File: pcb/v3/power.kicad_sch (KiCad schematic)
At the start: 51 parts, among them J6 Conn_01x02, J7 Conn_01x02, J8 Conn_01x03, J9 Conn_01x02, Q1 NPN, Q2 NPN, Q3 PMOS, U2 LM27762, U3 SY6918QDC, U5 LP5912-3.3DRV

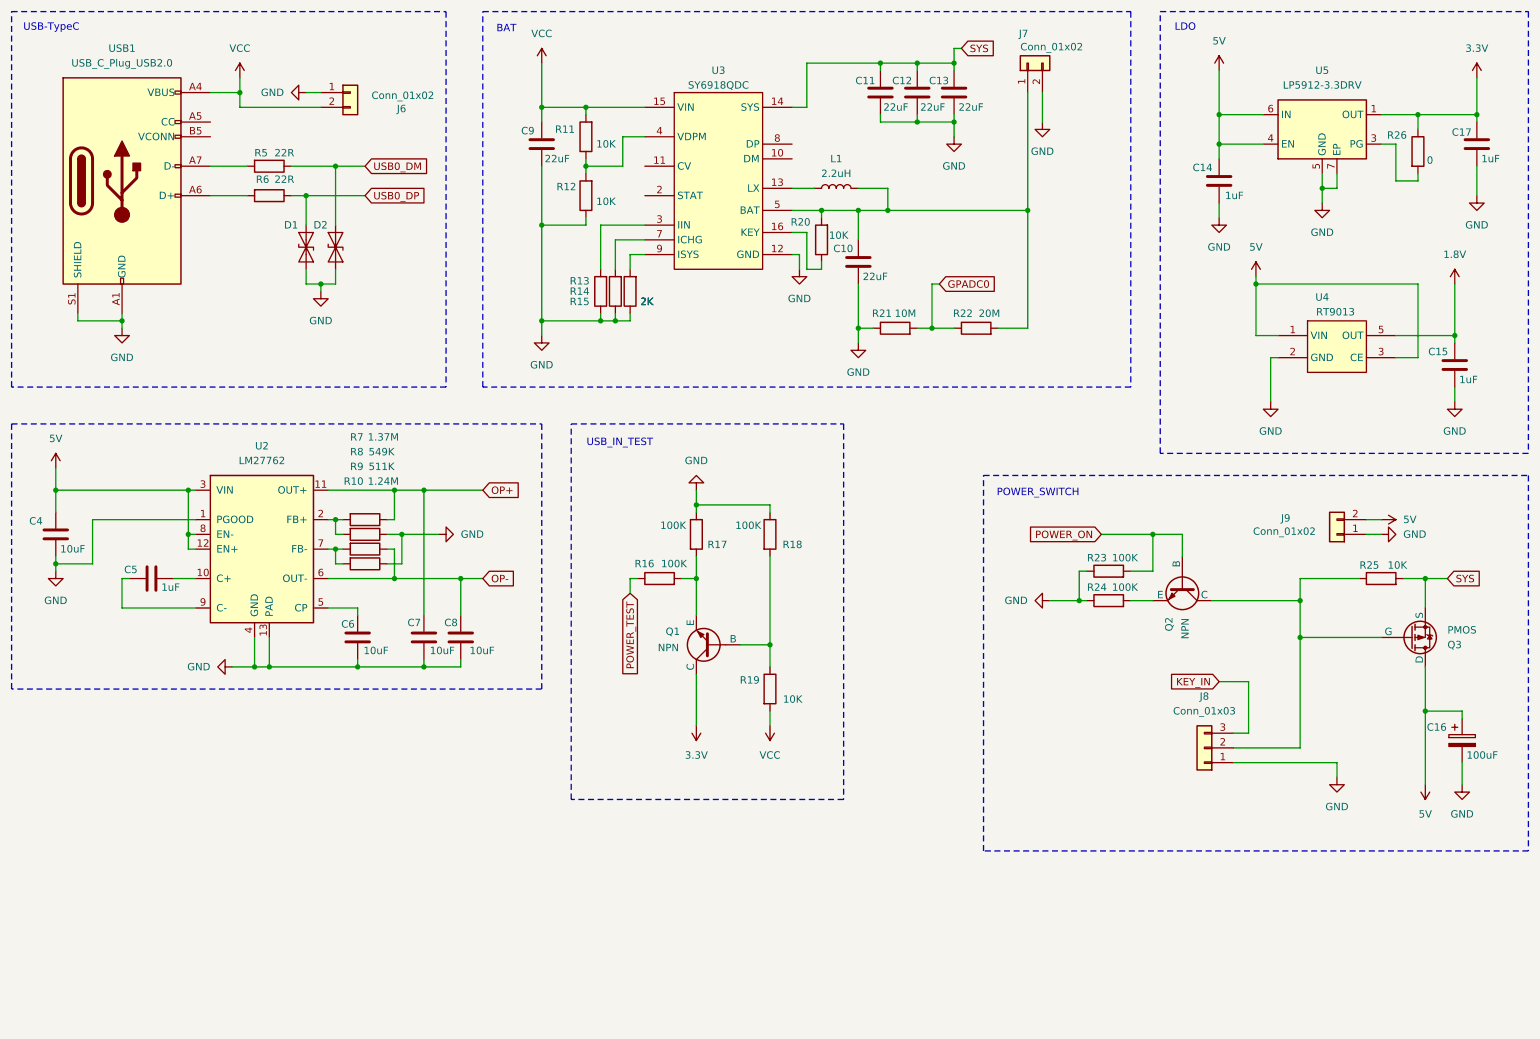
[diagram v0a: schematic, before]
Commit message: up
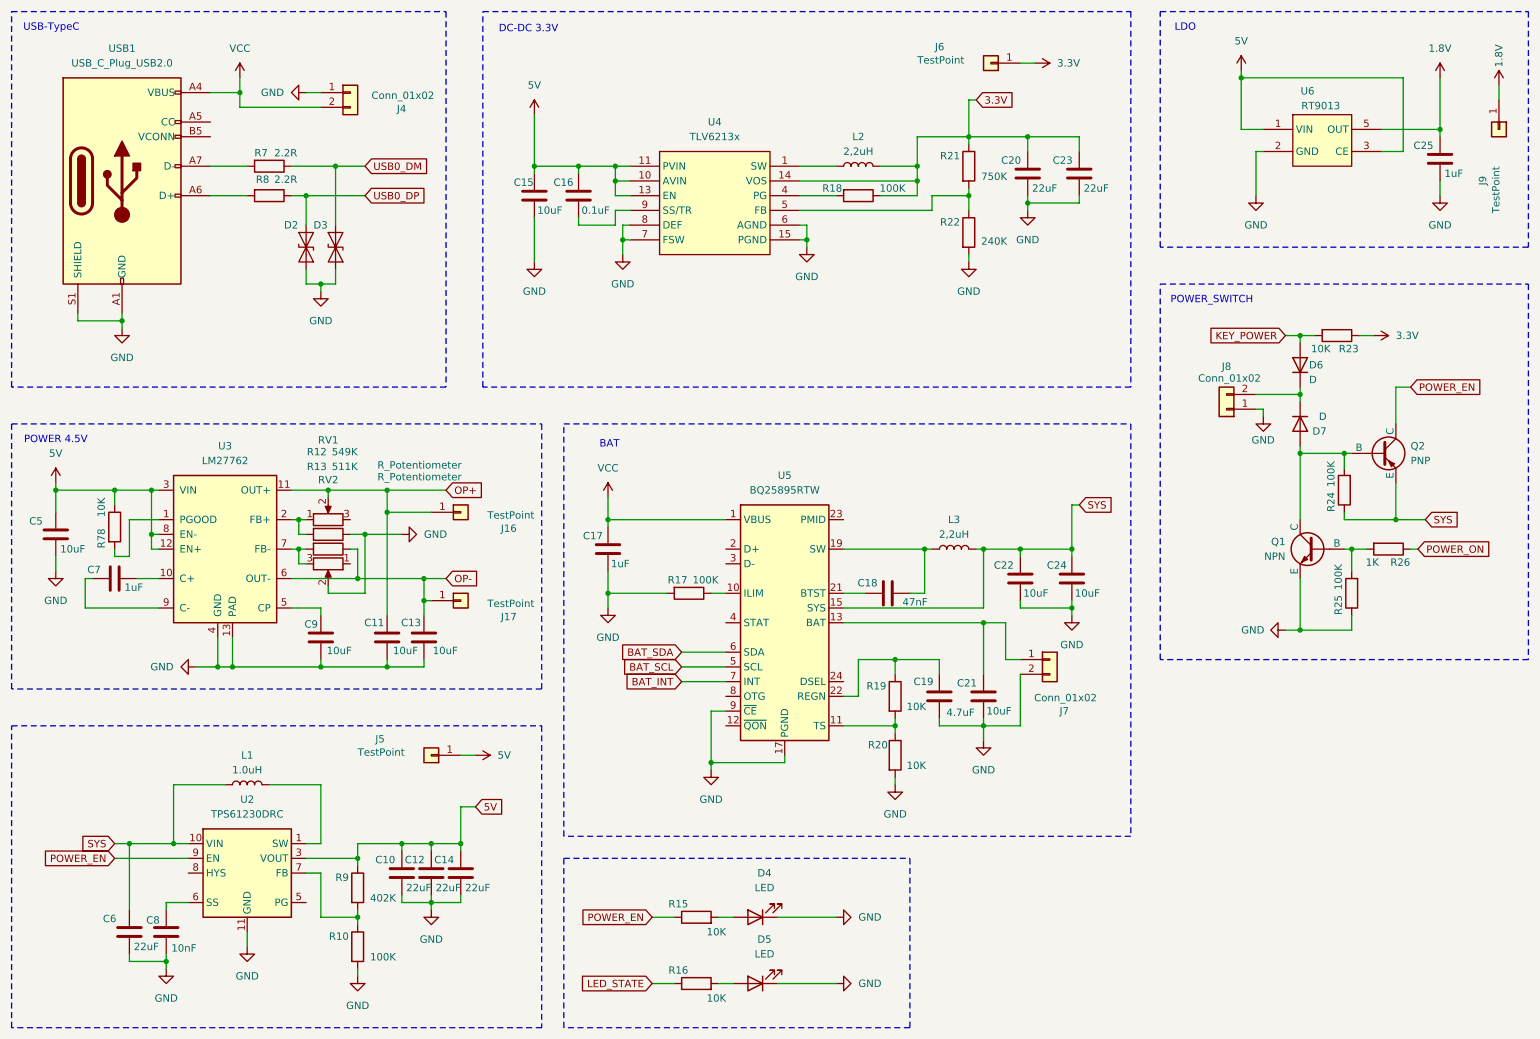
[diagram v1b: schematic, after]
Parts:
- removed C11, C13: 22uF, Capacitor_SMD:C_0603_1608Metric_Pad1.08x0.95mm_HandSolder, symbol Device:C
- removed C16: 100uF, Capacitor_Tantalum_SMD:CP_EIA-3528-21_Kemet-B_Pad1.50x2.35mm_HandSolder, symbol Device:C_Polarized
- removed Q2: NPN, Package_TO_SOT_SMD:SOT-23, symbol Simulation_SPICE:NPN
- removed Q3: PMOS, Package_TO_SOT_SMD:SOT-23_Handsoldering, symbol Simulation_SPICE:PMOS
- removed R11, R12: 10K, Capacitor_SMD:C_0402_1005Metric_Pad0.74x0.62mm_HandSolder, symbol Device:R
- removed R13, R14: 2K, Capacitor_SMD:C_0402_1005Metric_Pad0.74x0.62mm_HandSolder, symbol Device:R
- removed R7: 1.37M, Capacitor_SMD:C_0402_1005Metric_Pad0.74x0.62mm_HandSolder, symbol Device:R
- removed U3: SY6918QDC, coloryr:SY6918, symbol coloryr:SY6918
- removed U5: LP5912-3.3DRV, Package_SON:WSON-6-1EP_2x2mm_P0.65mm_EP1x1.6mm_ThermalVias, symbol Regulator_Linear:LP5912-3.3DRV
- added C16: 0.1uF, Capacitor_SMD:C_0402_1005Metric_Pad0.74x0.62mm_HandSolder, symbol Device:C
- added C18: 47nF, Capacitor_SMD:C_0402_1005Metric_Pad0.74x0.62mm_HandSolder, symbol Device:C
- added C19: 4.7uF, Capacitor_SMD:C_0402_1005Metric_Pad0.74x0.62mm_HandSolder, symbol Device:C
- added C20, C23: 22uF, Capacitor_SMD:C_0603_1608Metric_Pad1.08x0.95mm_HandSolder, symbol Device:C
- added C21, C22, C24: 10uF, Capacitor_SMD:C_0402_1005Metric_Pad0.74x0.62mm_HandSolder, symbol Device:C
- added C6: 22uF, Capacitor_SMD:C_0402_1005Metric_Pad0.74x0.62mm_HandSolder, symbol Device:C
- added C8: 10nF, Capacitor_SMD:C_0402_1005Metric_Pad0.74x0.62mm_HandSolder, symbol Device:C
- added D4, D5: LED, Diode_SMD:D_0402_1005Metric_Pad0.77x0.64mm_HandSolder, symbol Device:LED
- added D6, D7: D, Diode_SMD:D_SOD-323_HandSoldering, symbol Device:D
- added J16, J17, J6, J9: TestPoint, TestPoint:TestPoint_Pad_D2.0mm, symbol Connector_Generic:Conn_01x01
- added L2, L3: 2,2uH, Inductor_SMD:L_1008_2520Metric_Pad1.43x2.20mm_HandSolder, symbol Device:L
- added Q2: PNP, coloryr:SOT-23, symbol Simulation_SPICE:PNP
- added R78: 10K, Capacitor_SMD:C_0402_1005Metric_Pad0.74x0.62mm_HandSolder, symbol Device:R
- added R9: 402K, Capacitor_SMD:C_0402_1005Metric_Pad0.74x0.62mm_HandSolder, symbol Device:R
- added RV1, RV2: R_Potentiometer, Potentiometer_THT:Potentiometer_Bourns_3296W_Vertical, symbol Device:R_Potentiometer
- added U2: TPS61230DRC, Package_SON:Texas_S-PVSON-N10_ThermalVias, symbol Regulator_Switching:TPS61230DRC
- added U4: TLV6213x, Package_DFN_QFN:VQFN-16-1EP_3x3mm_P0.5mm_EP1.68x1.68mm_ThermalVias, symbol coloryr:TLV62130x
- added U5: BQ25895RTW, Package_DFN_QFN:Texas_RTW_WQFN-24-1EP_4x4mm_P0.5mm_EP2.7x2.7mm_ThermalVias, symbol Battery_Management:BQ25895RTW
- C14: value 1uF -> 22uF; footprint Capacitor_SMD:C_0402_1005Metric_Pad0.74x0.62mm_HandSolder -> Capacitor_SMD:C_0603_1608Metric_Pad1.08x0.95mm_HandSolder
- C15: renamed from C9; value 22uF -> 10uF; footprint Capacitor_SMD:C_0603_1608Metric_Pad1.08x0.95mm_HandSolder -> Capacitor_SMD:C_0402_1005Metric_Pad0.74x0.62mm_HandSolder
- J5: renamed from J9; value Conn_01x02 -> TestPoint; footprint Connector_PinHeader_2.54mm:PinHeader_1x02_P2.54mm_Vertical -> TestPoint:TestPoint_Pad_D2.0mm; symbol Connector_Generic:Conn_01x02 -> Connector_Generic:Conn_01x01
- J8: value Conn_01x03 -> Conn_01x02; footprint Connector_PinHeader_2.00mm:PinHeader_1x03_P2.00mm_Vertical -> Connector_PinHeader_2.00mm:PinHeader_1x02_P2.00mm_Vertical; symbol Connector_Generic:Conn_01x03 -> Connector_Generic:Conn_01x02
- L1: value 2.2uH -> 1.0uH; footprint Inductor_SMD:L_1008_2520Metric_Pad1.43x2.20mm_HandSolder -> Inductor_SMD:L_Changjiang_FXL0530
- Q1: footprint Package_TO_SOT_SMD:SOT-23 -> coloryr:SOT-23
- R10: value 1.24M -> 100K
- R15: value 2K -> 10K
- R16, R23: value 100K -> 10K
- R21: value 10M -> 750K; footprint Resistor_SMD:R_0402_1005Metric_Pad0.72x0.64mm_HandSolder -> Capacitor_SMD:C_0402_1005Metric_Pad0.74x0.62mm_HandSolder
- R22: value 20M -> 240K; footprint Inductor_SMD:L_0402_1005Metric_Pad0.77x0.64mm_HandSolder -> Capacitor_SMD:C_0402_1005Metric_Pad0.74x0.62mm_HandSolder
- R25: value 10K -> 100K
- R26: value 0 -> 1K
- R7: renamed from R5; value 22R -> 2.2R
- R8: renamed from R6; value 22R -> 2.2R
- renumbered C7 to C11, C8 to C13, C15 to C25, C4 to C5, C5 to C7, C6 to C9, D1 to D2, D2 to D3, J6 to J4, R8 to R12, R9 to R13, U2 to U3, U4 to U6
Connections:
- net 1.8V: now also J9.1 (Pin_1)
- net 3.3V: now also R18.1, R21.1, R23.1, C20.1, C23.1, J6.1 (Pin_1), L2.2, U4.14 (VOS); no longer C17.1, Q1.3 (C), R26.1
- net 5V: now also C10.1, C12.1, C15.1, J5.1 (Pin_1), C16.1, R78.1, R9.1, U2.3 (VOUT), U2.4 (VOUT), U4.10 (AVIN), U4.11 (PVIN), U4.12 (PVIN), U4.13 (EN); no longer J5.2 (Pin_2)
- net GND: now also Q1.3 (E), R10.2, R17.2, R20.2, R22.2, R25.1, C19.1, C20.2, C21.2, C22.2, C23.2, C24.2, C6.2, C8.1, D4.1 (K), D5.1 (K), RV2.2, U2.11 (GND), U4.15 (PGND), U4.16 (PGND), U4.17 (TAP), U4.6 (AGND), U4.7 (FSW), U4.8 (DEF), U5.17 (PGND), U5.18 (PGND), U5.25 (PGND), U5.9 (~{CE}); no longer J5.1 (Pin_1), R10.1, R15.1, R17.1, R18.1, R21.1, R23.1, R24.1, U3.1 (PGOOD)
- net OP+: now also J16.1 (Pin_1), RV1.2
- net OP-: now also J17.1 (Pin_1)
- net POWER_ON: now also R26.1; no longer R23.2
- net SYS: now also L1.1, R24.1, C22.1, C24.1, C6.1, L3.2, Q2.3 (E), U2.10 (VIN), U5.15 (SYS), U5.16 (SYS); no longer C12.1, R25.2
- net VCC: now also C17.1, U5.1 (VBUS); no longer C15.1, R19.2
- net at R26.2: now also Q1.2 (B), R25.2
- net at R13.2, U3.7 (FB-): now also RV2.3; no longer R10.2
- net at R12.2, U3.2 (FB+): now also RV1.1
- net at J8.2 (Pin_2): now also D6.1 (K), D7.1 (K); no longer R25.1
- net at R20.1: now also R19.2, U5.11 (TS)
- net at R15.2: now also D4.2 (A)
- net at R24.2: now also Q1.1 (C), D7.2 (A), Q2.2 (B)
- net GPADC0: no longer names the net of R21.2, R22.1
- net GPADC0: now also U4.5 (FB)
- removed net KEY_IN: J8.3 (Pin_3)
- net POWER_TEST renamed LED_STATE
- new net: D5.2 (A), R16.2
- new net: C18.1, U5.21 (BTST)
- new net: C18.2, L3.1, U5.19 (SW), U5.20 (SW)
- new net: R17.1, U5.10 (ILIM)
- new net: L2.1, U4.1 (SW), U4.2 (SW), U4.3 (SW)
- new net: R18.2, U4.4 (PG)
- new net: C16.2, U4.9 (SS/TR)
- new net: C19.2, R19.1, U5.22 (REGN)
- new net: R10.1, R9.2, U2.7 (FB)
- new net: C8.2, U2.6 (SS)
- new net: L1.2, U2.1 (SW), U2.2 (SW)
- new net: C21.1, J7.1 (Pin_1), U5.13 (BAT), U5.14 (BAT)
- new net: R78.2, U3.1 (PGOOD)
- new net BAT_INT: U5.7 (INT)
- new net BAT_SCL: U5.5 (SCL)
- new net BAT_SDA: U5.6 (SDA)
- new net KEY_POWER: D6.2 (A), R23.2
- new net POWER_EN: Q2.1 (C), R15.1, U2.9 (EN)
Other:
- note added: "DC-DC 3.3V"
- note added: "POWER 4.5V"
- note removed: "USB_IN_TEST"
- moved on the sheet: C11, C13, C15, C25, C7, C9, R12, R13, R24, U3, U6
